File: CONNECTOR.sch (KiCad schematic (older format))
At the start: 13 parts, among them J2 QTH-030-02-L-DA, U7 SN74AUP1G06DCKR, U8 SN74AUP1G07DCKR, U9 SN74AUP1G06DCKR

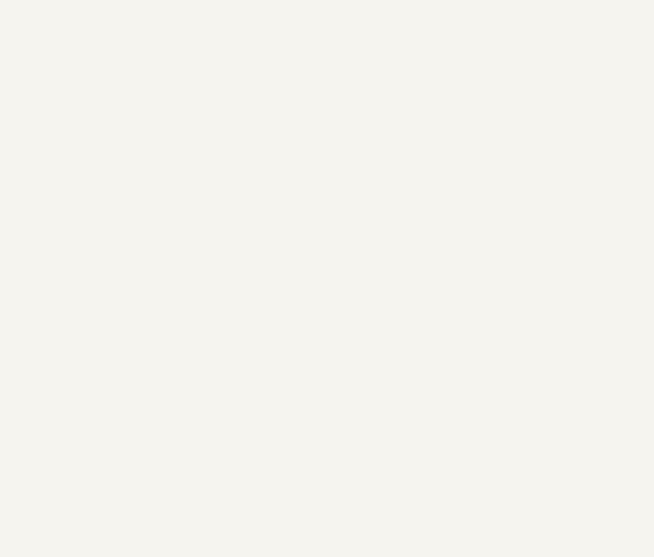
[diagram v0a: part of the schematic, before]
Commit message: First Final -- Waiting for Checker
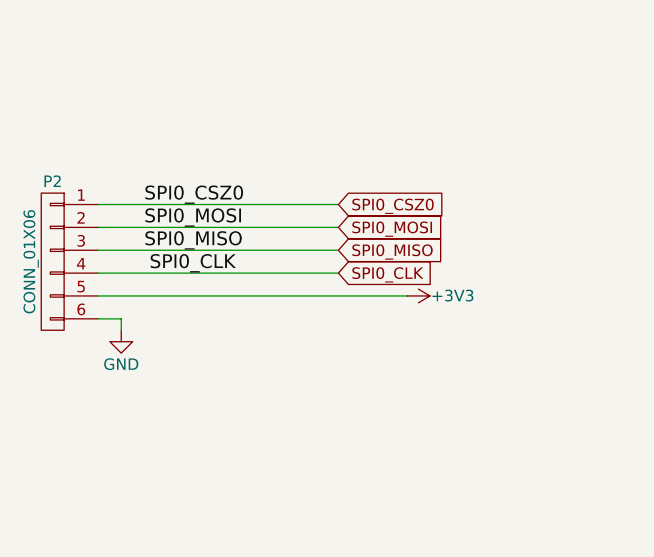
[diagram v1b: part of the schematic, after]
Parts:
- added P2: CONN_01X06, Pin_Headers:Pin_Header_Straight_1x06, symbol CONN_01X06
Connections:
- net +3V3: now also P2.5 (P5)
- net GND: now also P2.6 (P6)
- net SPI0_CLK: now also P2.4 (P4)
- net SPI0_CSZ0: now also P2.1 (P1)
- net SPI0_MISO: now also P2.3 (P3)
- net SPI0_MOSI: now also P2.2 (P2)
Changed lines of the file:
@@
 $EndComp
 $Comp
-L SYSPWR #PWR20
+L SYSPWR #PWR22
 U 1 1 56F83223
 P 6500 6100
-F 0 "#PWR20" H 6550 6050 100 0001 C CNN
+F 0 "#PWR22" H 6550 6050 100 0001 C CNN
 F 1 "SYSPWR" V 6500 6350 50  0000 C CNN
 F 2 "" H 6500 6100 100 0000 C CNN
@@
 Connection ~ 11700 8850
 $Comp
-L SYSPWR #PWR22
+L SYSPWR #PWR24
 U 1 1 56F9621E
 P 9000 6100
-F 0 "#PWR22" H 9050 6050 100 0001 C CNN
+F 0 "#PWR24" H 9050 6050 100 0001 C CNN
 F 1 "SYSPWR" V 9000 6350 50  0000 C CNN
 F 2 "" H 9000 6100 100 0000 C CNN
@@
 	0    1    1    0
 $EndComp
+$Comp
+L CONN_01X06 P2
+U 1 1 56FD0D03
+P 1500 3700
+F 0 "P2" H 1500 4050 50  0000 C CNN
+F 1 "CONN_01X06" V 1600 3700 50  0000 C CNN
+F 2 "Pin_Headers:Pin_Header_Straight_1x06" H 1500 3700 60  0001 C CNN
+F 3 "" H 1500 3700 60  0000 C CNN
+	1    1500 3700
+	-1   0    0    -1
+$EndComp
+Text GLabel 2750 3650 2    50   Input ~ 0
+SPI0_MISO
+Text GLabel 2750 3550 2    50   Input ~ 0
+SPI0_MOSI
+Text GLabel 2750 3450 2    50   Input ~ 0
+SPI0_CSZ0
+Wire Wire Line
+	2750 3450 1700 3450
+Wire Wire Line
+	2750 3550 1700 3550
+Text Label 1900 3650 0    60   ~ 0
+SPI0_MISO
+Text Label 1900 3550 0    60   ~ 0
+SPI0_MOSI
+Text Label 1900 3450 0    60   ~ 0
+SPI0_CSZ0
+Wire Wire Line
+	2750 3650 1700 3650
+Text GLabel 2750 3750 2    50   Input ~ 0
+SPI0_CLK
+Wire Wire Line
+	2750 3750 1700 3750
+Text Label 2300 3750 2    60   ~ 0
+SPI0_CLK
+$Comp
+L +3V3 #PWR030
+U 1 1 56FD15FD
+P 3050 3850
+F 0 "#PWR030" H 3050 3700 50  0001 C CNN
+F 1 "+3V3" V 3050 4050 50  0000 C CNN
+F 2 "" H 3050 3850 60  0000 C CNN
+F 3 "" H 3050 3850 60  0000 C CNN
+	1    3050 3850
+	0    1    1    0
+$EndComp
+Wire Wire Line
+	1700 3850 3050 3850
+$Comp
+L GND #PWR031
+U 1 1 56FD175C
+P 1800 4000
+F 0 "#PWR031" H 1800 3750 50  0001 C CNN
+F 1 "GND" H 1800 3850 50  0000 C CNN
+F 2 "" H 1800 4000 60  0000 C CNN
+F 3 "" H 1800 4000 60  0000 C CNN
+	1    1800 4000
+	1    0    0    -1
+$EndComp
+Wire Wire Line
+	1700 3950 1800 3950
+Wire Wire Line
+	1800 3950 1800 4000
 $EndSCHEMATC
